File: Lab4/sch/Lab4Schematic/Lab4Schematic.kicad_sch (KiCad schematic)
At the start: 3 parts, among them SW1 CK_KMS2xxG, U1 2478, U2 Pico

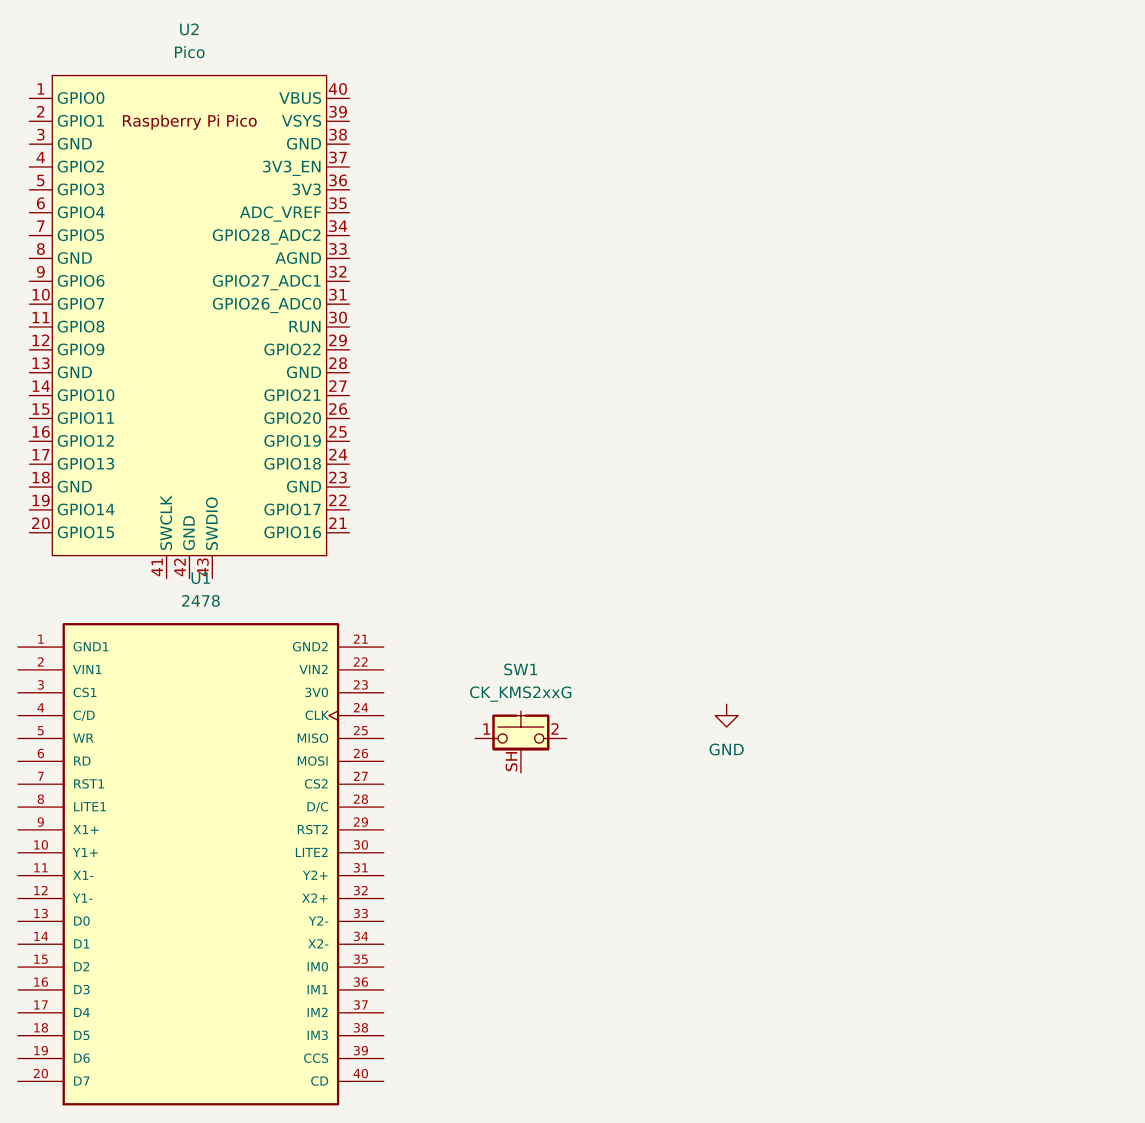
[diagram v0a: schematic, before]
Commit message: schematic created
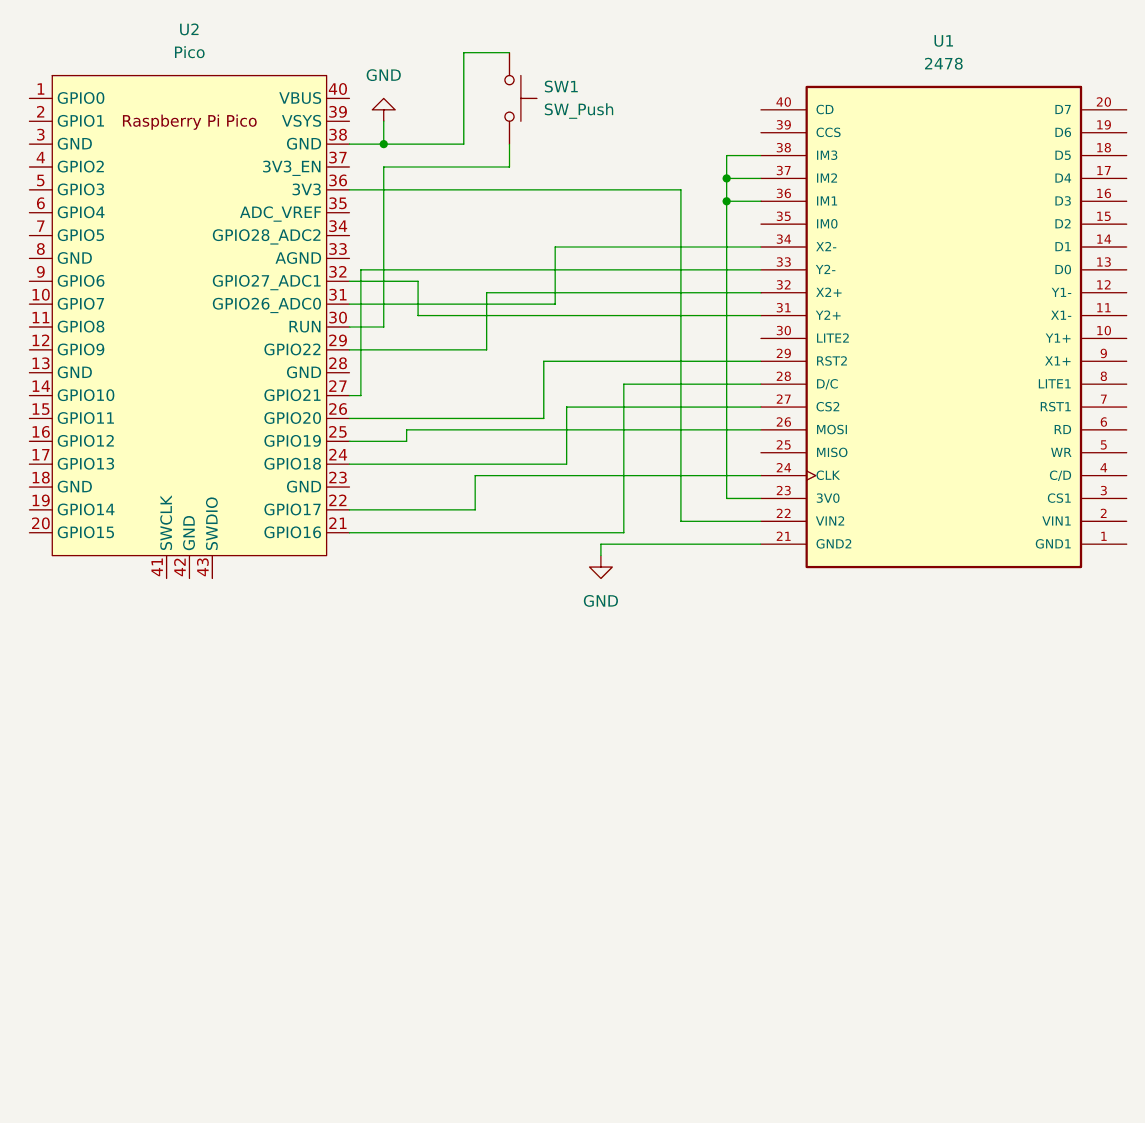
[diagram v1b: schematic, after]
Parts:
- removed SW1: CK_KMS2xxG, Button_Switch_SMD:SW_SPST_CK_KMS2xxGP, symbol Switch:CK_KMS2xxG
- added SW1: SW_Push, symbol Switch:SW_Push
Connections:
- net GND: now also U1.21 (GND2), U2.38 (GND), SW1.1
- net at U1.22 (VIN2): now also U2.36 (3V3)
- net at U1.23 (3V0): now also U1.36 (IM1), U1.37 (IM2), U1.38 (IM3)
- net at U1.24 (CLK): now also U2.22 (GPIO17)
- net at U1.26 (MOSI): now also U2.25 (GPIO19)
- net at U1.27 (CS2): now also U2.24 (GPIO18)
- net at U1.28 (D/C): now also U2.21 (GPIO16)
- net at U1.29 (RST2): now also U2.26 (GPIO20)
- net at U1.31 (Y2+): now also U2.32 (GPIO27_ADC1)
- net at U1.32 (X2+): now also U2.29 (GPIO22)
- net at U1.33 (Y2-): now also U2.27 (GPIO21)
- net at U1.34 (X2-): now also U2.31 (GPIO26_ADC0)
- net at U2.30 (RUN): now also SW1.2
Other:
- company: (none) -> Lafayette College
- title: (none) -> Lab 4 Schematic - Pico and LCD Touchscreen
